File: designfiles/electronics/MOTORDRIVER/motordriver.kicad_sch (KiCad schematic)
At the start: 0 parts

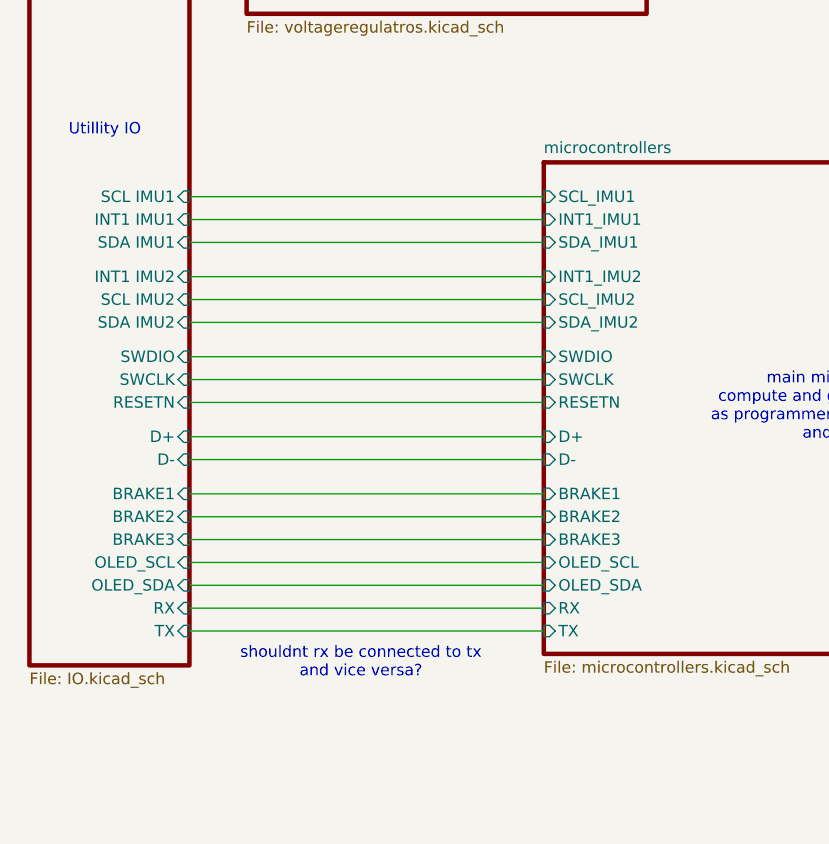
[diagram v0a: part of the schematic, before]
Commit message: worked on PCB
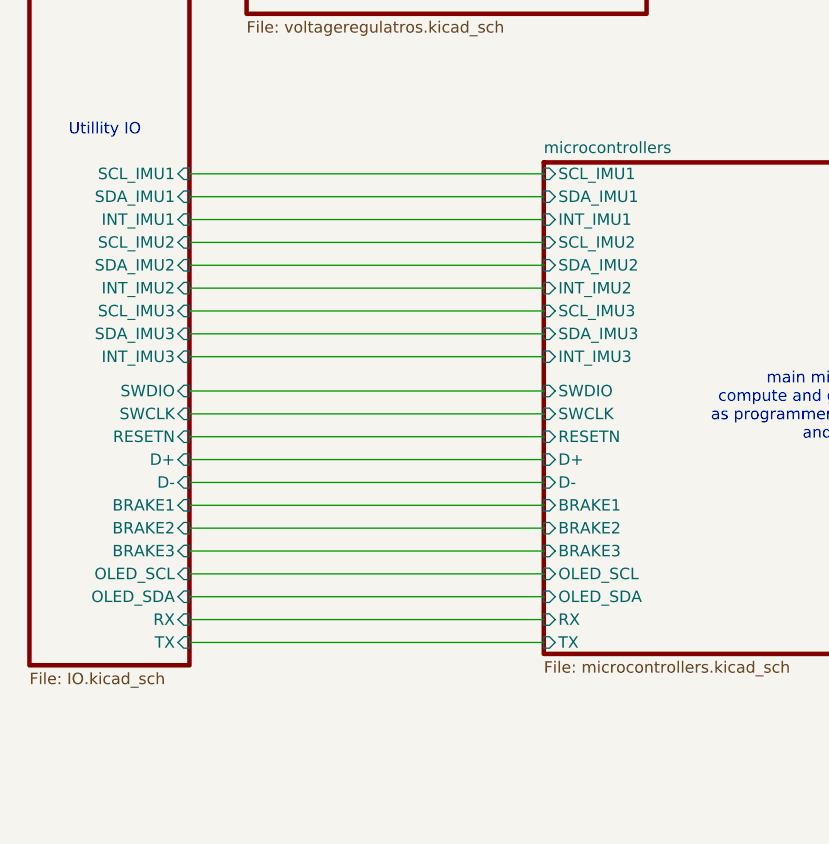
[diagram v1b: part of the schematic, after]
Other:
- sheet IO ports: added INT_IMU1, INT_IMU2, INT_IMU3, SCL_IMU1, SCL_IMU2, SCL_IMU3, SDA_IMU1, SDA_IMU2, SDA_IMU3; removed INT1 IMU1, INT1 IMU2, SCL IMU1, SCL IMU2, SDA IMU1, SDA IMU2
- sheet microcontrollers ports: added INT_IMU1, INT_IMU2, INT_IMU3, SCL_IMU3, SDA_IMU3; removed INT1_IMU1, INT1_IMU2
- note removed: "shouldnt rx be connected to tx and vice versa?"
